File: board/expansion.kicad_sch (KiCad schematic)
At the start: 2 parts, among them U13 ENGINE

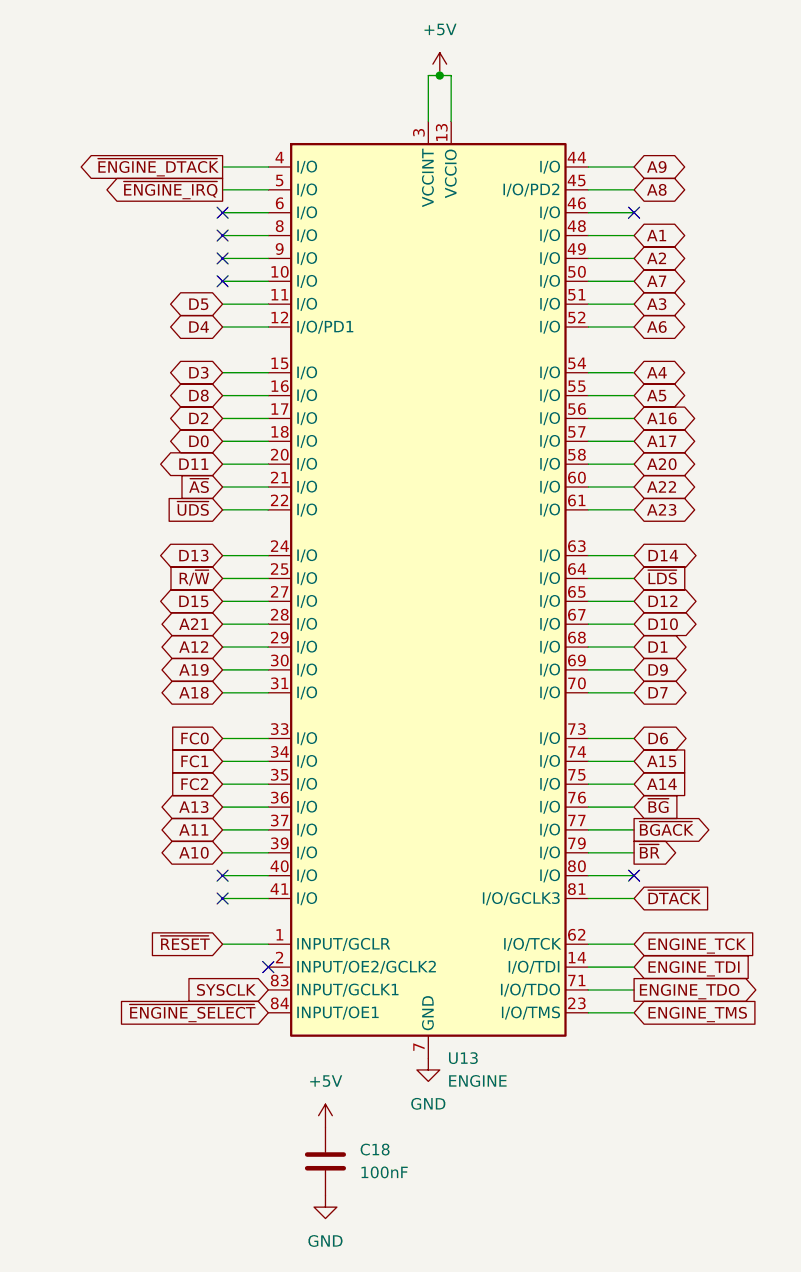
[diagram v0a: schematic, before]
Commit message: checkpoint
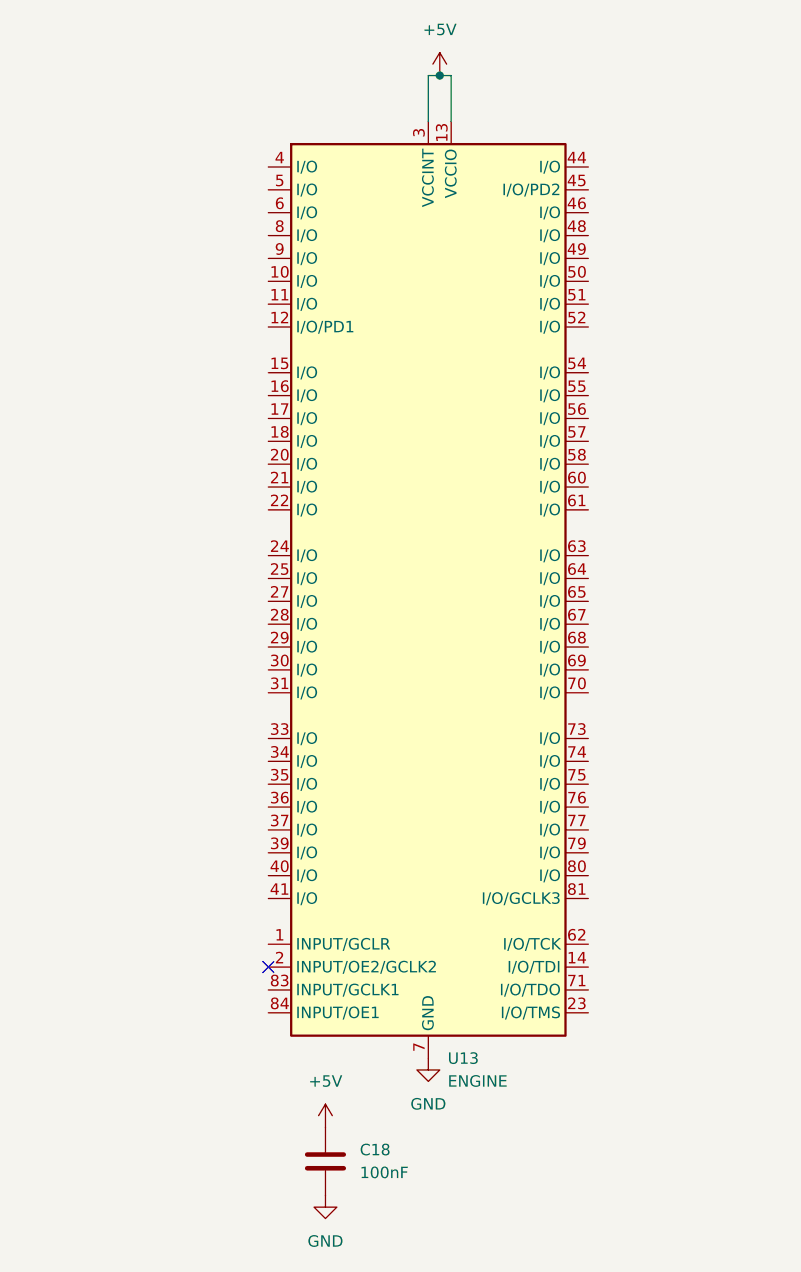
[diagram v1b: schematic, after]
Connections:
- net A1: no longer names the net of U13.48 (I/O)
- net A10: no longer names the net of U13.39 (I/O)
- net A11: no longer names the net of U13.37 (I/O)
- net A12: no longer names the net of U13.29 (I/O)
- net A13: no longer names the net of U13.36 (I/O)
- net A14: no longer names the net of U13.75 (I/O)
- net A15: no longer names the net of U13.74 (I/O)
- net A16: no longer names the net of U13.56 (I/O)
- net A17: no longer names the net of U13.57 (I/O)
- net A18: no longer names the net of U13.31 (I/O)
- net A19: no longer names the net of U13.30 (I/O)
- net A2: no longer names the net of U13.49 (I/O)
- net A20: no longer names the net of U13.58 (I/O)
- net A21: no longer names the net of U13.28 (I/O)
- net A22: no longer names the net of U13.60 (I/O)
- net A23: no longer names the net of U13.61 (I/O)
- net A3: no longer names the net of U13.51 (I/O)
- net A4: no longer names the net of U13.54 (I/O)
- net A5: no longer names the net of U13.55 (I/O)
- net A6: no longer names the net of U13.52 (I/O)
- net A7: no longer names the net of U13.50 (I/O)
- net A8: no longer names the net of U13.45 (I/O/PD2)
- net A9: no longer names the net of U13.44 (I/O)
- net D0: no longer names the net of U13.18 (I/O)
- net D1: no longer names the net of U13.68 (I/O)
- net D10: no longer names the net of U13.67 (I/O)
- net D11: no longer names the net of U13.20 (I/O)
- net D12: no longer names the net of U13.65 (I/O)
- net D13: no longer names the net of U13.24 (I/O)
- net D14: no longer names the net of U13.63 (I/O)
- net D15: no longer names the net of U13.27 (I/O)
- net D2: no longer names the net of U13.17 (I/O)
- net D3: no longer names the net of U13.15 (I/O)
- net D4: no longer names the net of U13.12 (I/O/PD1)
- net D5: no longer names the net of U13.11 (I/O)
- net D6: no longer names the net of U13.73 (I/O)
- net D7: no longer names the net of U13.70 (I/O)
- net D8: no longer names the net of U13.16 (I/O)
- net D9: no longer names the net of U13.69 (I/O)
- net ENGINE_TCK: no longer names the net of U13.62 (I/O/TCK)
- net ENGINE_TDI: no longer names the net of U13.14 (I/O/TDI)
- net ENGINE_TDO: no longer names the net of U13.71 (I/O/TDO)
- net ENGINE_TMS: no longer names the net of U13.23 (I/O/TMS)
- net FC0: no longer names the net of U13.33 (I/O)
- net FC1: no longer names the net of U13.34 (I/O)
- net FC2: no longer names the net of U13.35 (I/O)
- net R/~{W}: no longer names the net of U13.25 (I/O)
- net SYSCLK: no longer names the net of U13.83 (INPUT/GCLK1)
- net ~{AS}: no longer names the net of U13.21 (I/O)
- net ~{BGACK}: no longer names the net of U13.77 (I/O)
- net ~{BG}: no longer names the net of U13.76 (I/O)
- net ~{BR}: no longer names the net of U13.79 (I/O)
- net ~{DTACK}: no longer names the net of U13.81 (I/O/GCLK3)
- net ~{ENGINE_DTACK}: no longer names the net of U13.4 (I/O)
- net ~{ENGINE_IRQ}: no longer names the net of U13.5 (I/O)
- net ~{ENGINE_SELECT}: no longer names the net of U13.84 (INPUT/OE1)
- net ~{LDS}: no longer names the net of U13.64 (I/O)
- net ~{RESET}: no longer names the net of U13.1 (INPUT/GCLR)
- net ~{UDS}: no longer names the net of U13.22 (I/O)
- no-connect marks 9 -> 1
